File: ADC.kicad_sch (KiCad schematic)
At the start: 162 parts, among them J1 Conn_01x03_Pin, J2 Screw_Terminal_01x02, J3 Screw_Terminal_01x09, SW1 SW_SPDT, U1 ADS1256IDBR, U10 CD4514BM, U11 ADG5412FBCPZ-RL7, U12 ADR421ARMZ, U13 OPA211ID, U14 ADG5412FBCPZ-RL7, U15 OPA211ID, U16 ADG5412FBCPZ-RL7, U17 OPA211ID, U19 CD4514BM, U2 MCU-STM32F407VET6_LQFP100_, U20 ADG5412FBCPZ-RL7, U21 ADG5412FBCPZ-RL7, U22 ADG5412FBCPZ-RL7, U23 ADG5412FBCPZ-RL7, U24 OPA211ID, U25 OPA211ID, U26 OPA211ID, U27 OPA211ID, U3 ADM2483xRW, U4 LM2596S-5, U5 DCP010505BP, U7 OPA211ID, U8 AMS1117-3.3, U9 ADG5412FBCPZ-RL7, Y1 8MHz, Y2 ABM3B-25.000MHZ-D2Y-T

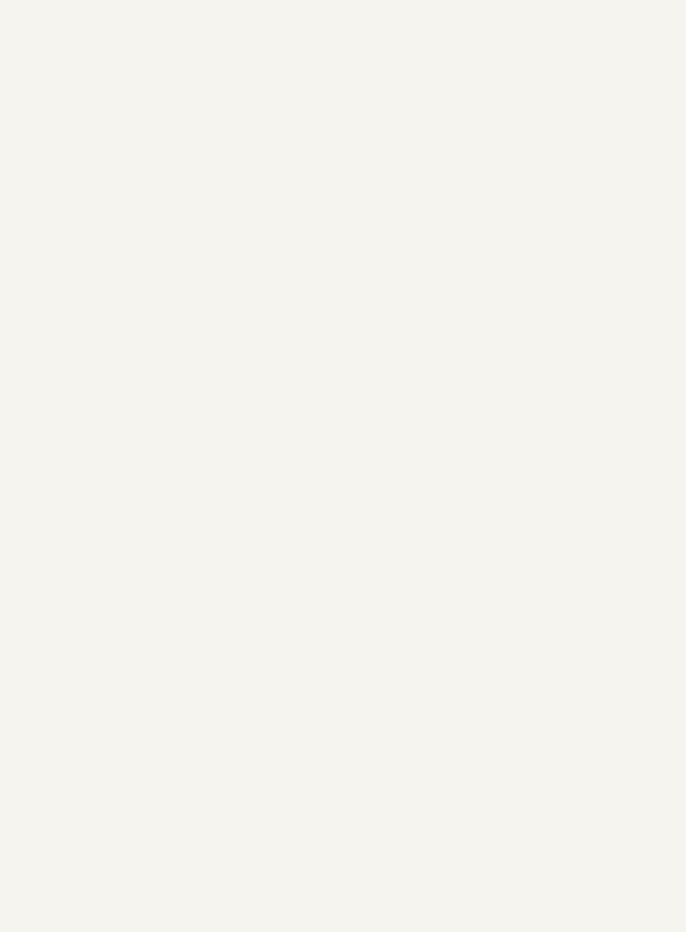
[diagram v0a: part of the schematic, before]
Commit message: Add TLV
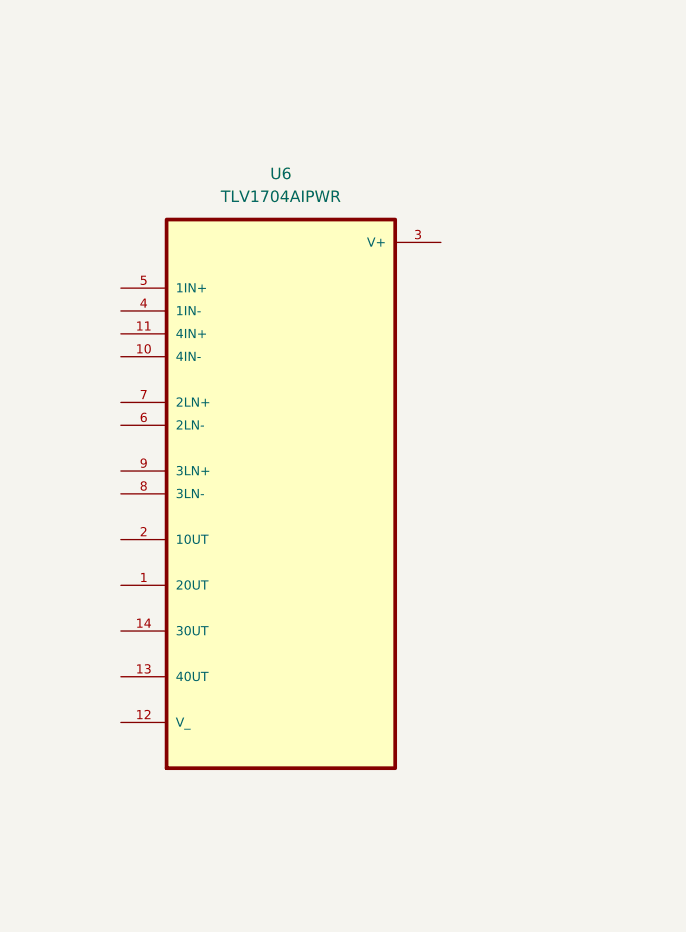
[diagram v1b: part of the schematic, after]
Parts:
- added U6: TLV1704AIPWR, TLV1704AIPWR:SOP65P640X120-14N, symbol TLV1704AIPWR:TLV1704AIPWR
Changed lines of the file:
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@@
+	)
+	(symbol
+		(lib_id "TLV1704AIPWR:TLV1704AIPWR")
+		(at 110.49 605.79 0)
+		(unit 1)
+		(exclude_from_sim no)
+		(in_bom yes)
+		(on_board yes)
+		(dnp no)
+		(fields_autoplaced yes)
+		(property "Reference" "U6"
+			(at 110.49 570.23 0)
+			(effects
+				(font
+					(size 1.27 1.27)
+				)
+			)
+		)
+		(property "Value" "TLV1704AIPWR"
+			(at 110.49 572.77 0)
+			(effects
+				(font
+					(size 1.27 1.27)
+				)
+			)
+		)
+		(property "Footprint" "TLV1704AIPWR:SOP65P640X120-14N"
+			(at 110.49 605.79 0)
+			(effects
+				(font
+					(size 1.27 1.27)
+				)
+				(justify bottom)
+				(hide yes)
+			)
+		)
+		(property "Datasheet" ""
+			(at 110.49 605.79 0)
+			(effects
+				(font
+					(size 1.27 1.27)
+				)
+				(hide yes)
+			)
+		)
+		(property "Description" ""
+			(at 110.49 605.79 0)
+			(effects
+				(font
+					(size 1.27 1.27)
+				)
+				(hide yes)
+			)
+		)
+		(property "MF" "Texas Instruments"
+			(at 110.49 605.79 0)
+			(effects
+				(font
+					(size 1.27 1.27)
+				)
+				(justify bottom)
+				(hide yes)
+			)
+		)
+		(property "Description_1" "\n                        \n                            Quad high voltage, low power comparator\n                        \n"
+			(at 110.49 605.79 0)
+			(effects
+				(font
+					(size 1.27 1.27)
+				)
+				(justify bottom)
+				(hide yes)
+			)
+		)
+		(property "Package" "TSSOP-14 Texas Instruments"
+			(at 110.49 605.79 0)
+			(effects
+				(font
+					(size 1.27 1.27)
+				)
+				(justify bottom)
+				(hide yes)
+			)
+		)
+		(property "Price" "None"
+			(at 110.49 605.79 0)
+			(effects
+				(font
+					(size 1.27 1.27)
+				)
+				(justify bottom)
+				(hide yes)
+			)
+		)
+		(property "SnapEDA_Link" "https://www.snapeda.com/parts/TLV1704AIPWR/Texas+Instruments/view-part/?ref=snap"
+			(at 110.49 605.79 0)
+			(effects
+				(font
+					(size 1.27 1.27)
+				)
+				(justify bottom)
+				(hide yes)
+			)
+		)
+		(property "MP" "TLV1704AIPWR"
+			(at 110.49 605.79 0)
+			(effects
+				(font
+					(size 1.27 1.27)
+				)
+				(justify bottom)
+				(hide yes)
+			)
+		)
+		(property "Availability" "In Stock"
+			(at 110.49 605.79 0)
+			(effects
+				(font
+					(size 1.27 1.27)
+				)
+				(justify bottom)
+				(hide yes)
+			)
+		)
+		(property "Check_prices" "https://www.snapeda.com/parts/TLV1704AIPWR/Texas+Instruments/view-part/?ref=eda"
+			(at 110.49 605.79 0)
+			(effects
+				(font
+					(size 1.27 1.27)
+				)
+				(justify bottom)
+				(hide yes)
+			)
+		)
+		(pin "5"
+		)
+		(pin "6"
+		)
+		(pin "13"
+		)
+		(pin "14"
+		)
+		(pin "12"
+		)
+		(pin "2"
+		)
+		(pin "3"
+		)
+		(pin "4"
+		)
+		(pin "1"
+		)
+		(pin "9"
+		)
+		(pin "8"
+		)
+		(pin "7"
+		)
+		(pin "11"
+		)
+		(pin "10"
+		)
+		(instances
+			(project ""
+				(path "/c7ceee6a-ba62-44b0-b5ba-f64f163625fc"
+					(reference "U6")
+					(unit 1)
+				)
+			)
+		)
 	)
 	(symbol
